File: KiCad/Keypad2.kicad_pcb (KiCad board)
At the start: 2 copper layers, 13.2 x 29 mm, 19 parts, among them J1 Keypad, J2 Prog, U1 SP3485, U2 ESP32-PICO-MINI-02, U3 LMR16006+FB, U4 QR

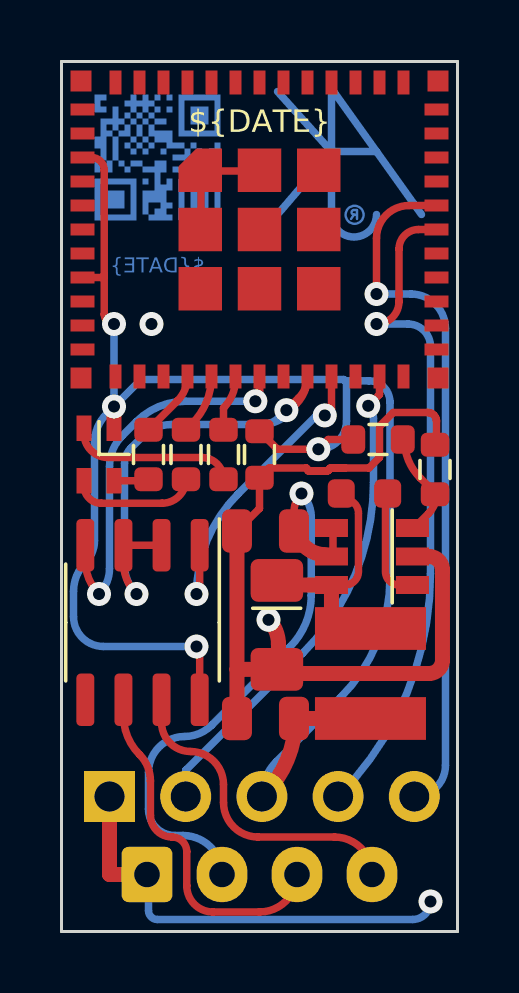
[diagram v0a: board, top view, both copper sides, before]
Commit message: C/R on EN
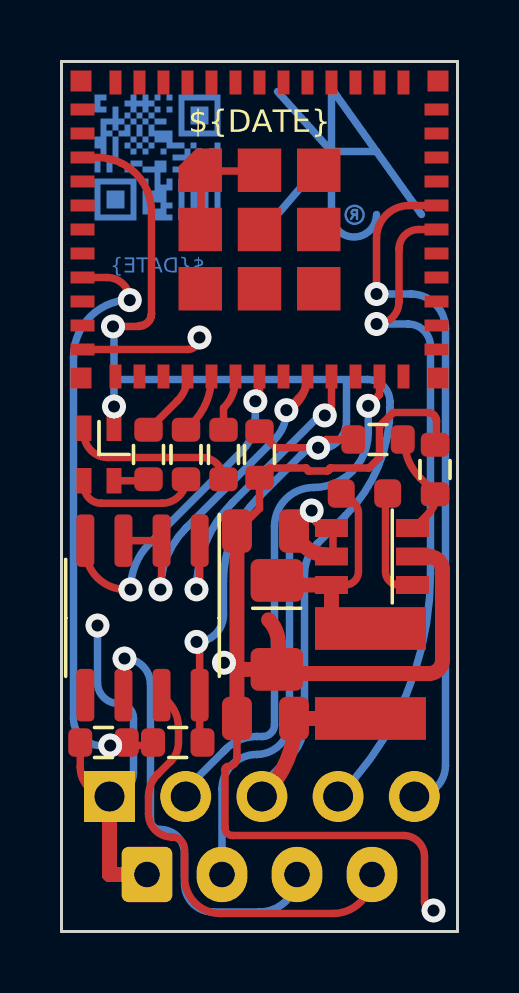
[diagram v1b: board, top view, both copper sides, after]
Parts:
- added C1: 10nF, RevK:C_0603, F.Cu at (162.4, 116.7)
- added R1: 10K, RevK:R_0603, F.Cu at (164.9, 116.7)
- moved U1 0.15 mm to (163.7, 112.5)
- renumbered C1 to C2, C2 to C3, C3 to C4, C4 to C5, R1 to R2, R2 to R3, R3 to R4, R4 to R5, R5 to R6
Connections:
- U2 pad 8: +3V3 -> Net-(C1-Pad2)
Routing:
- net Net-(C1-Pad2): track 0.00 -> 20.1 mm, vias 0 -> 2
- net GND: track 32.2 -> 52.0 mm, vias 3 -> 4
- net DE: track 17.0 -> 12.8 mm
- net Net-(J1-Pad4): track 10.7 -> 14.8 mm
- net +12V: track 19.0 -> 15.6 mm
- net Net-(J1-Pad3): track 11.9 -> 14.7 mm, vias 0 -> 1
- net TX: track 13.8 -> 11.5 mm
- net GPIO0: track 16.4 -> 17.5 mm
- net +3V3: track 58.0 -> 57.0 mm
